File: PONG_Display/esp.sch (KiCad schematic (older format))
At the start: 2 parts, among them J7 ESP_Conn, J8 ESP_Prog_Conn

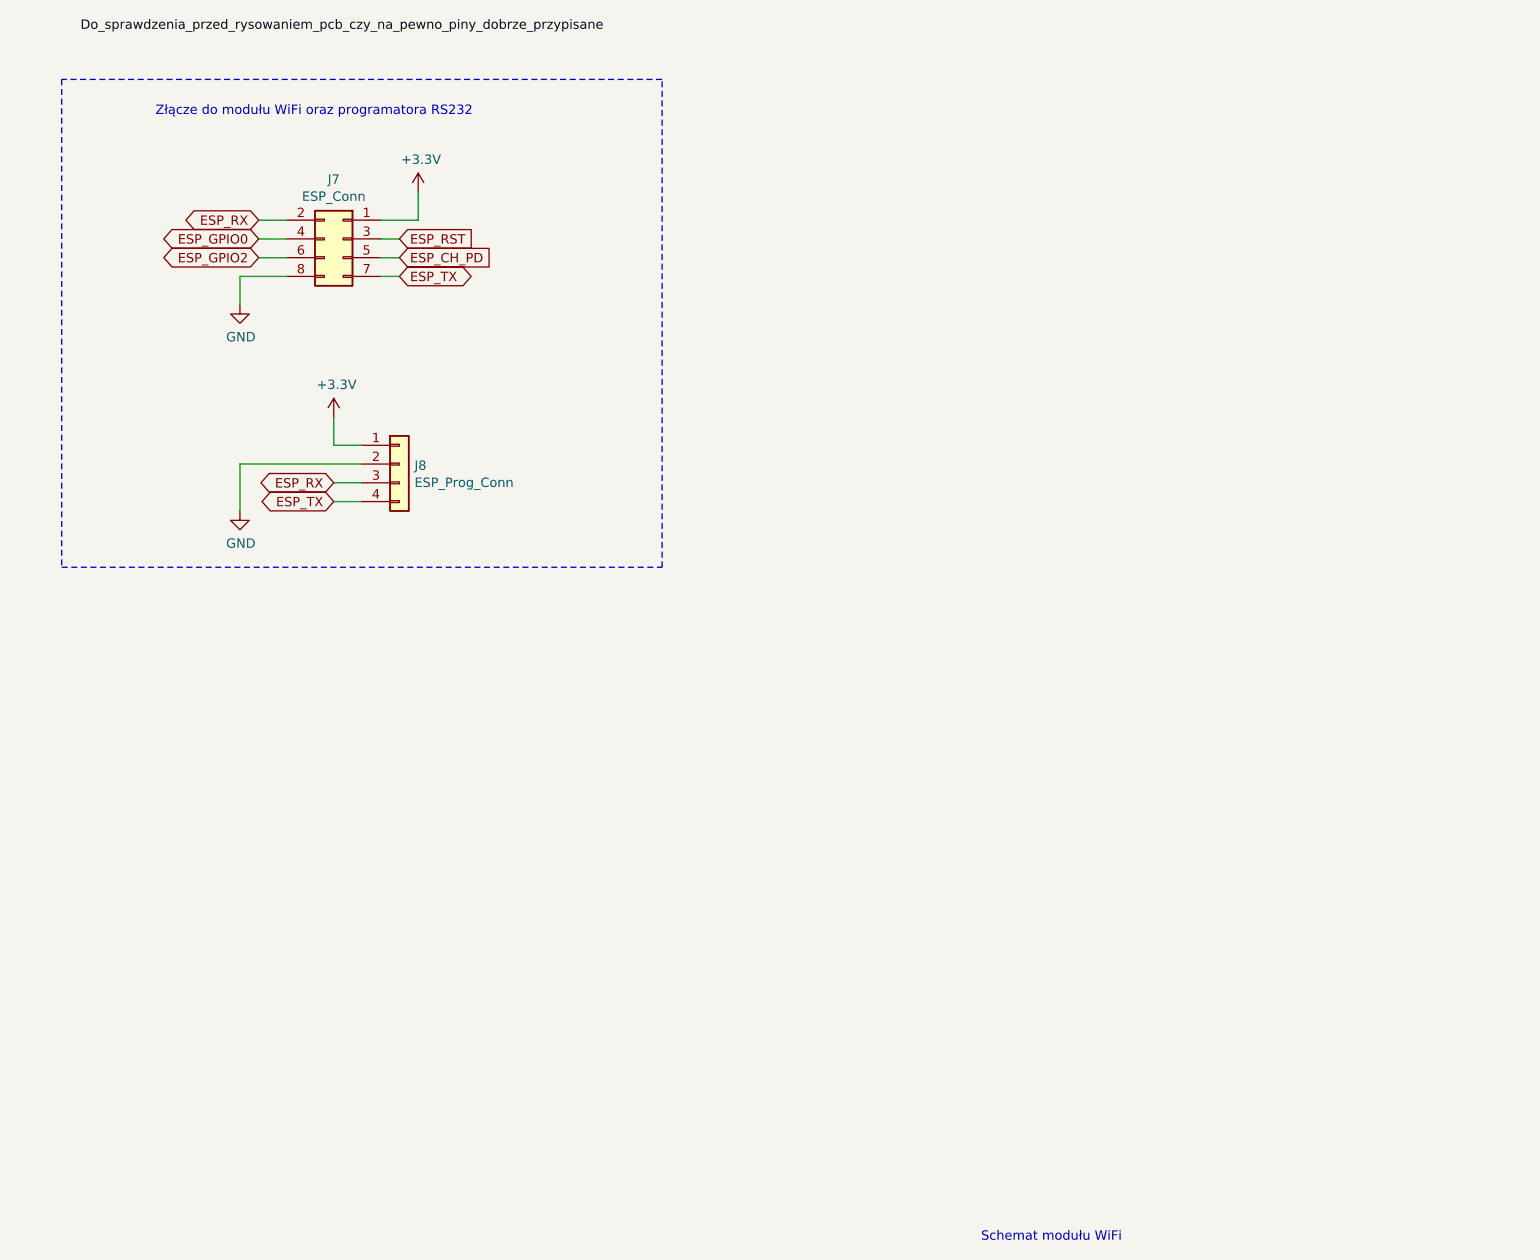
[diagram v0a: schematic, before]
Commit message: Zmiany
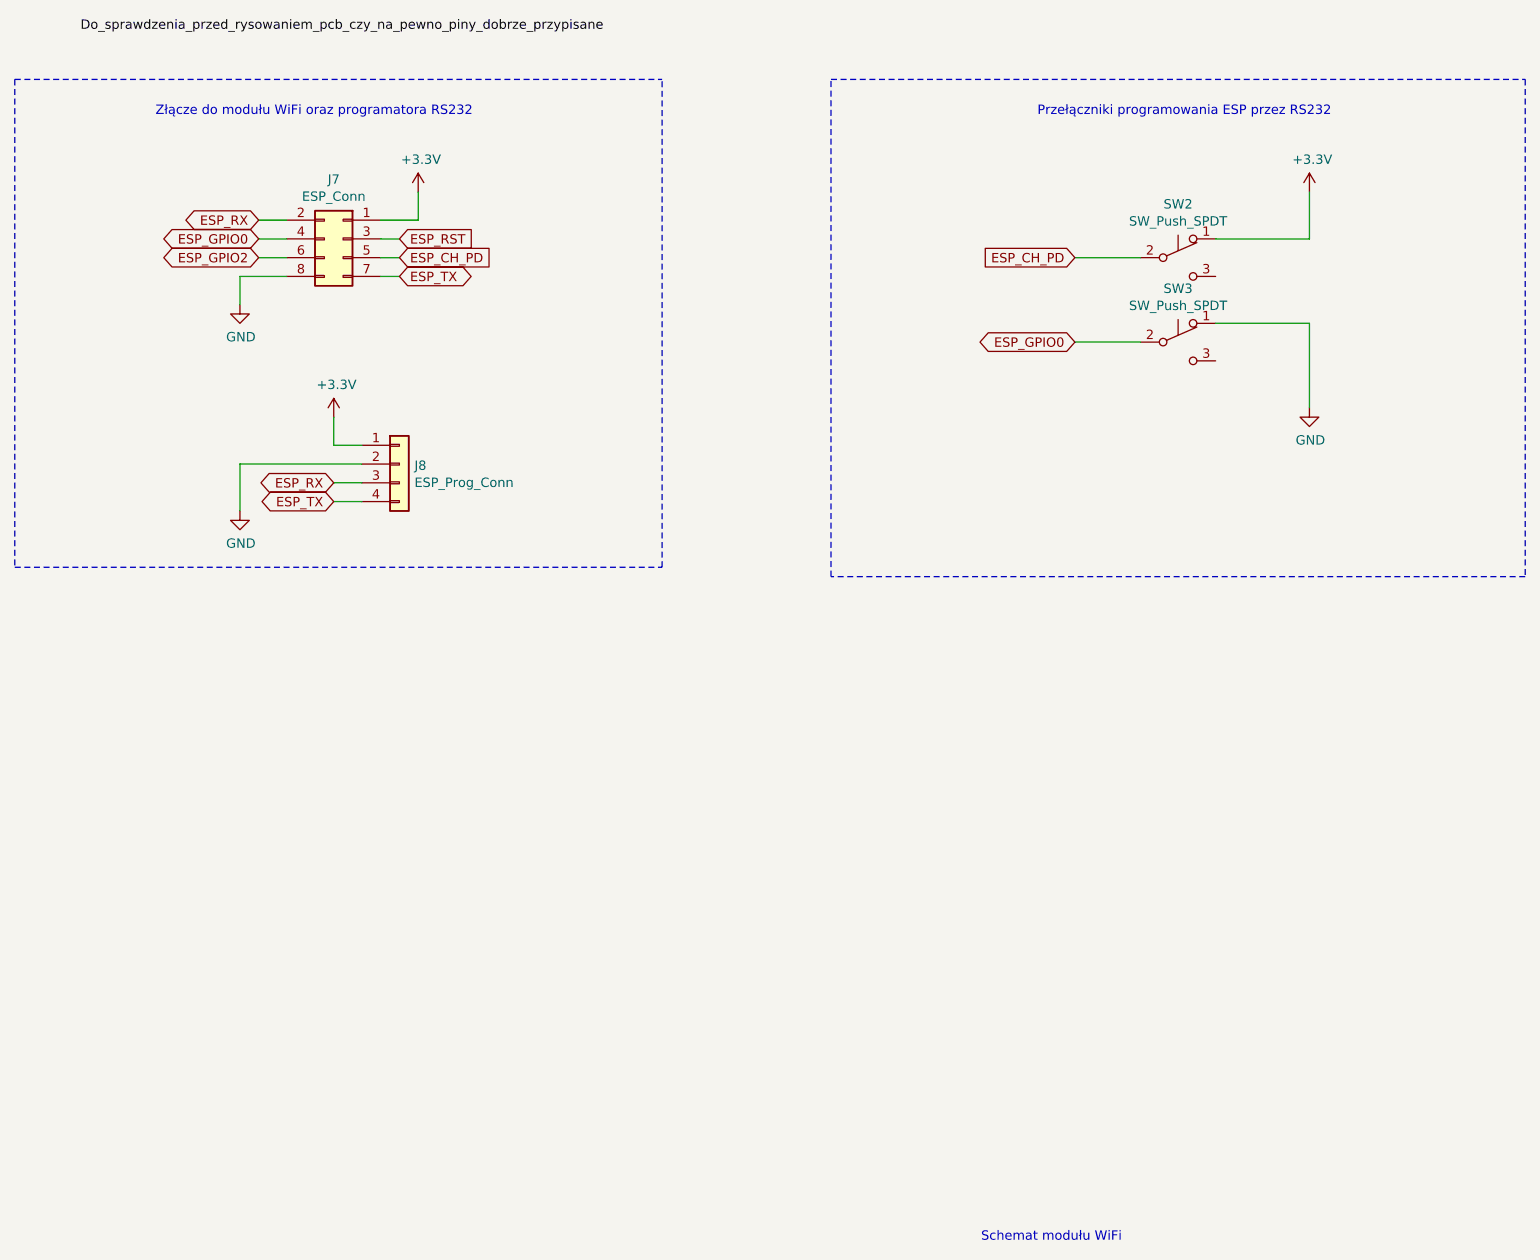
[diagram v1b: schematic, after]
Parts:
- added SW2, SW3: SW_Push_SPDT, LIB_PONG_Display:SPDT_switch, symbol Switch:SW_Push_SPDT
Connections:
- net +3V3: now also SW2.1 (A)
- net ESP_CH_PD: now also SW2.2 (B)
- net ESP_GPIO0: now also SW3.2 (B)
- net GND: now also SW3.1 (A)
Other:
- note added: "Przełączniki programowania ESP przez RS232"
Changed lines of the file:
@@
 	3850 3350 4500 3350
-Wire Notes Line
-	2900 3900 6100 3900
 Wire Notes Line
 	6100 3900 6100 1300
 Wire Notes Line
-	6100 1300 2900 1300
-Wire Notes Line
-	2900 1300 2900 3900
+	2650 1300 2650 3900
 Text Notes 3400 1500 0    50   ~ 0
 Złącze do modułu WiFi oraz programatora RS232
 Text Label 3000 1050 0    50   ~ 0
 Do_sprawdzenia_przed_rysowaniem_pcb_czy_na_pewno_piny_dobrze_przypisane
+Wire Notes Line
+	2650 1300 6100 1300
+Wire Notes Line
+	2650 3900 6100 3900
+Wire Notes Line
+	10700 1300 10700 3950
+Wire Notes Line
+	10700 3950 7000 3950
+Wire Notes Line
+	7000 3950 7000 1300
+Wire Notes Line
+	7000 1300 10700 1300
+Text Notes 8100 1500 0    50   ~ 0
+Przełączniki programowania ESP przez RS232
+Text GLabel 8300 2250 0    50   Input ~ 0
+ESP_CH_PD
+Text GLabel 8300 2700 0    50   BiDi ~ 0
+ESP_GPIO0
+$Comp
+L power:+3.3V #PWR01
+U 1 1 5E9D6E89
+P 9550 1900
+F 0 "#PWR01" H 9550 1750 50  0001 C CNN
+F 1 "+3.3V" H 9565 2073 50  0000 C CNN
+F 2 "" H 9550 1900 50  0001 C CNN
+F 3 "" H 9550 1900 50  0001 C CNN
+	1    9550 1900
+	1    0    0    -1
+$EndComp
+$Comp
+L power:GND #PWR02
+U 1 1 5E9D779A
+P 9550 3050
+F 0 "#PWR02" H 9550 2800 50  0001 C CNN
+F 1 "GND" H 9555 2877 50  0000 C CNN
+F 2 "" H 9550 3050 50  0001 C CNN
+F 3 "" H 9550 3050 50  0001 C CNN
+	1    9550 3050
+	1    0    0    -1
+$EndComp
+Wire Wire Line
+	9550 1900 9550 2150
+Wire Wire Line
+	9550 2150 9050 2150
+Wire Wire Line
+	9050 2600 9550 2600
+Wire Wire Line
+	9550 2600 9550 3050
+Wire Wire Line
+	8300 2250 8650 2250
+Wire Wire Line
+	8300 2700 8650 2700
+$Comp
+L Switch:SW_Push_SPDT SW2
+U 1 1 5E9E35EF
+P 8850 2250
+F 0 "SW2" H 8850 2535 50  0000 C CNN
+F 1 "SW_Push_SPDT" H 8850 2444 50  0000 C CNN
+F 2 "LIB_PONG_Display:SPDT_switch" H 8850 2250 50  0001 C CNN
+F 3 "~" H 8850 2250 50  0001 C CNN
+	1    8850 2250
+	1    0    0    -1
+$EndComp
+$Comp
+L Switch:SW_Push_SPDT SW3
+U 1 1 5E9E3E9D
+P 8850 2700
+F 0 "SW3" H 8850 2985 50  0000 C CNN
+F 1 "SW_Push_SPDT" H 8850 2894 50  0000 C CNN
+F 2 "LIB_PONG_Display:SPDT_switch" H 8850 2700 50  0001 C CNN
+F 3 "~" H 8850 2700 50  0001 C CNN
+	1    8850 2700
+	1    0    0    -1
+$EndComp
 $EndSCHEMATC

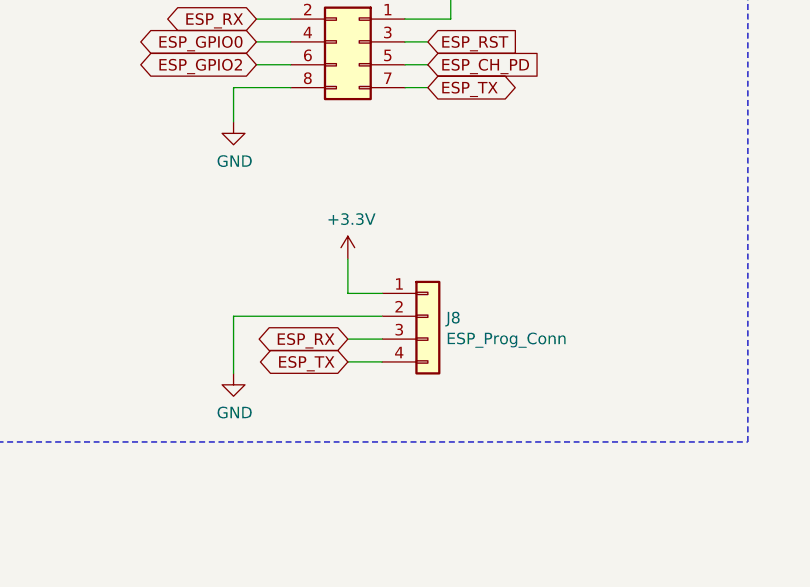
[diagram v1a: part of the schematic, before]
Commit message: Zmiana
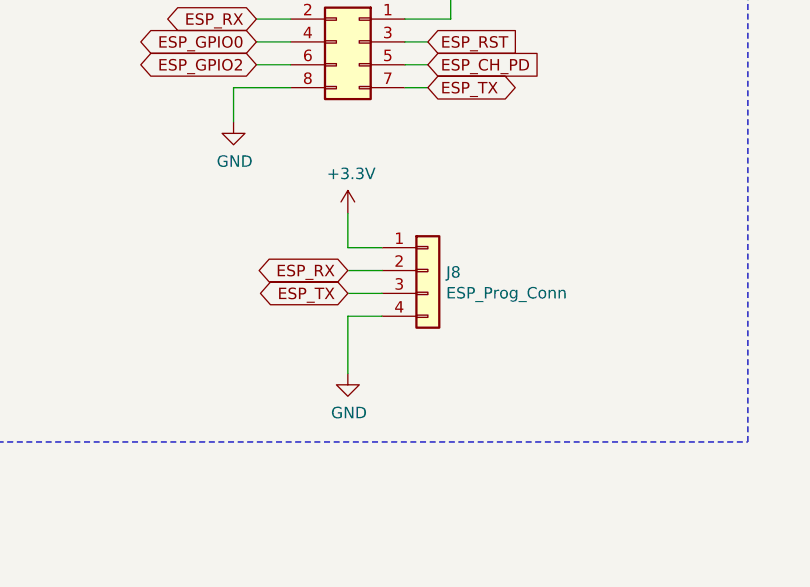
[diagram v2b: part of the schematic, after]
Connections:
- net ESP_RX: now also J8.2 (Pin_2); no longer J8.3 (Pin_3)
- net ESP_TX: now also J8.3 (Pin_3); no longer J8.4 (Pin_4)
- net GND: now also J8.4 (Pin_4); no longer J8.2 (Pin_2)
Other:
- moved on the sheet: J8
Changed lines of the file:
@@
 L Connector_Generic:Conn_01x04 J?
 U 1 1 5E838282
-P 4700 3350
+P 4700 3150
 AR Path="/5E80CCDD/5E838282" Ref="J?"  Part="1"
 AR Path="/5E80B1F8/5E838282" Ref="J8"  Part="1"
-F 0 "J8" H 4780 3342 50  0000 L CNN
-F 1 "ESP_Prog_Conn" H 4780 3251 50  0000 L CNN
-F 2 "Connector_PinHeader_2.54mm:PinHeader_1x04_P2.54mm_Vertical" H 4700 3350 50  0001 C CNN
-F 3 "~" H 4700 3350 50  0001 C CNN
-	1    4700 3350
+F 0 "J8" H 4780 3142 50  0000 L CNN
+F 1 "ESP_Prog_Conn" H 4780 3051 50  0000 L CNN
+F 2 "Connector_PinHeader_2.54mm:PinHeader_1x04_P2.54mm_Vertical" H 4700 3150 50  0001 C CNN
+F 3 "~" H 4700 3150 50  0001 C CNN
+	1    4700 3150
 	1    0    0    -1
 $EndComp
 Wire Wire Line
+	4350 3050 4500 3050
+Wire Wire Line
+	4350 3150 4500 3150
+Wire Wire Line
 	4350 3250 4500 3250
-Wire Wire Line
-	4350 3450 4500 3450
-Wire Wire Line
-	4350 3550 4500 3550
-Text GLabel 4350 3550 0    50   BiDi ~ 0
+Text GLabel 4350 3250 0    50   BiDi ~ 0
 ESP_TX
-Text GLabel 4350 3450 0    50   BiDi ~ 0
+Text GLabel 4350 3150 0    50   BiDi ~ 0
 ESP_RX
 Text Notes 7800 7500 0    50   ~ 0
@@
 L power:+3.3V #PWR0175
 U 1 1 5E859CE6
-P 4350 3100
-F 0 "#PWR0175" H 4350 2950 50  0001 C CNN
-F 1 "+3.3V" H 4365 3273 50  0000 C CNN
-F 2 "" H 4350 3100 50  0001 C CNN
-F 3 "" H 4350 3100 50  0001 C CNN
-	1    4350 3100
+P 4350 2900
+F 0 "#PWR0175" H 4350 2750 50  0001 C CNN
+F 1 "+3.3V" H 4365 3073 50  0000 C CNN
+F 2 "" H 4350 2900 50  0001 C CNN
+F 3 "" H 4350 2900 50  0001 C CNN
+	1    4350 2900
 	1    0    0    -1
 $EndComp
@@
 L power:GND #PWR0176
 U 1 1 5E85A6F5
-P 3850 3600
-F 0 "#PWR0176" H 3850 3350 50  0001 C CNN
-F 1 "GND" H 3855 3427 50  0000 C CNN
-F 2 "" H 3850 3600 50  0001 C CNN
-F 3 "" H 3850 3600 50  0001 C CNN
-	1    3850 3600
+P 4350 3600
+F 0 "#PWR0176" H 4350 3350 50  0001 C CNN
+F 1 "GND" H 4355 3427 50  0000 C CNN
+F 2 "" H 4350 3600 50  0001 C CNN
+F 3 "" H 4350 3600 50  0001 C CNN
+	1    4350 3600
 	1    0    0    -1
 $EndComp
 Wire Wire Line
-	4350 3100 4350 3250
+	4350 2900 4350 3050
 Wire Wire Line
-	3850 3350 3850 3600
+	4350 3350 4350 3600
 Wire Wire Line
-	3850 3350 4500 3350
+	4350 3350 4500 3350
 Wire Notes Line
 	6100 3900 6100 1300

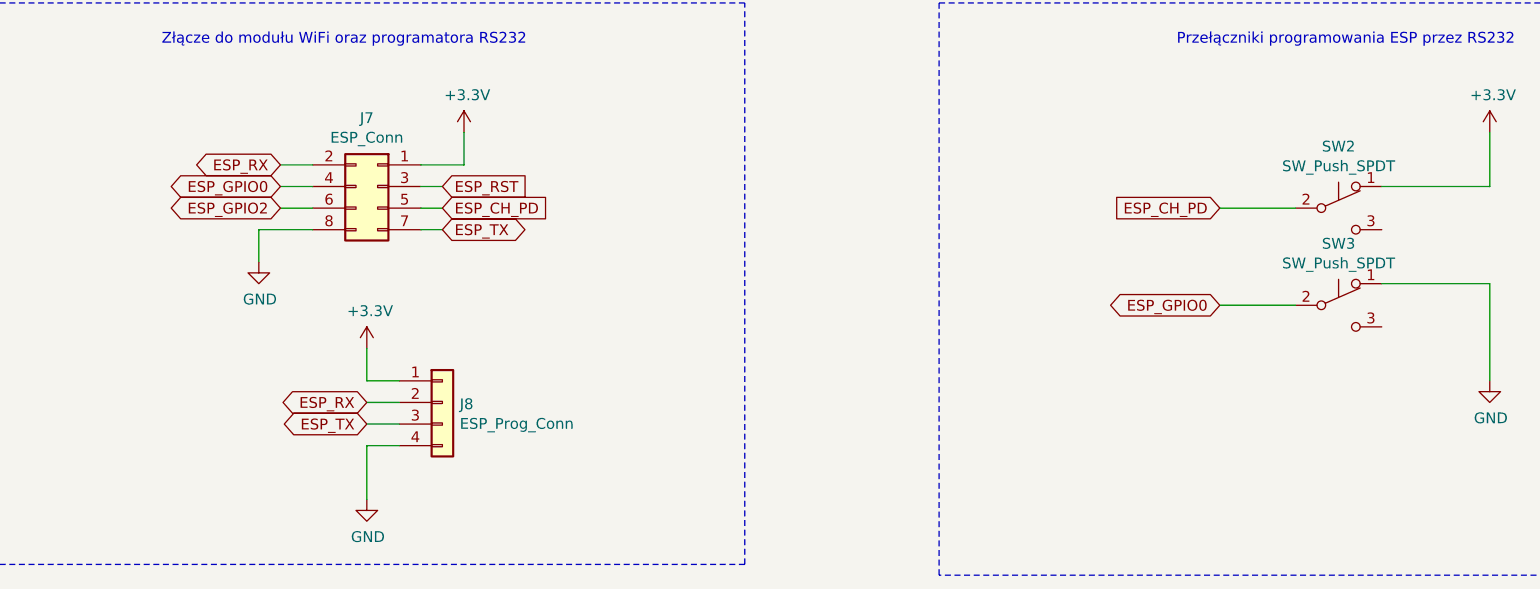
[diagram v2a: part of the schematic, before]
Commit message: Teraz jest sexy
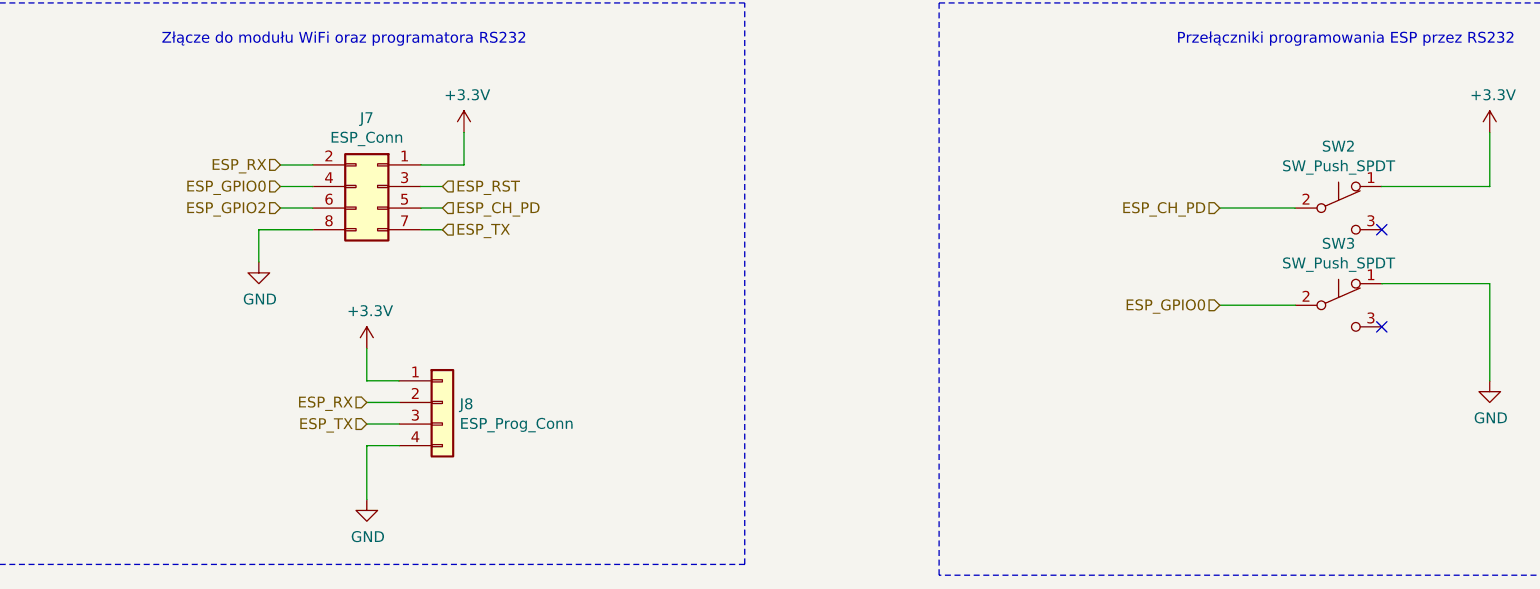
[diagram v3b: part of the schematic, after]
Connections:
- no-connect marks 0 -> 2
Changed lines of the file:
@@
 EESchema Schematic File Version 4
+LIBS:PONG_Display-cache
 EELAYER 30 0
 EELAYER END
@@
 Comment4 ""
 $EndDescr
-Text GLabel 4700 2150 2    50   Input ~ 0
-ESP_RST
-Text GLabel 4700 2250 2    50   Input ~ 0
-ESP_CH_PD
-Text GLabel 4700 2350 2    50   BiDi ~ 0
-ESP_TX
-Text GLabel 3950 2050 0    50   BiDi ~ 0
-ESP_RX
-Text GLabel 3950 2150 0    50   BiDi ~ 0
-ESP_GPIO0
-Text GLabel 3950 2250 0    50   BiDi ~ 0
-ESP_GPIO2
 $Comp
 L Connector_Generic:Conn_02x04_Odd_Even J?
@@
 Wire Wire Line
 	4350 3250 4500 3250
-Text GLabel 4350 3250 0    50   BiDi ~ 0
-ESP_TX
-Text GLabel 4350 3150 0    50   BiDi ~ 0
-ESP_RX
 Text Notes 7800 7500 0    50   ~ 0
 Schemat modułu WiFi
@@
 Text Notes 8100 1500 0    50   ~ 0
 Przełączniki programowania ESP przez RS232
-Text GLabel 8300 2250 0    50   Input ~ 0
-ESP_CH_PD
-Text GLabel 8300 2700 0    50   BiDi ~ 0
-ESP_GPIO0
 $Comp
 L power:+3.3V #PWR01
@@
 	1    0    0    -1
 $EndComp
+Text HLabel 3950 2050 0    50   Input ~ 0
+ESP_RX
+Text HLabel 4700 2350 2    50   Input ~ 0
+ESP_TX
+Text HLabel 4700 2150 2    50   Input ~ 0
+ESP_RST
+Text HLabel 4700 2250 2    50   Input ~ 0
+ESP_CH_PD
+Text HLabel 3950 2150 0    50   Input ~ 0
+ESP_GPIO0
+Text HLabel 3950 2250 0    50   Input ~ 0
+ESP_GPIO2
+Text HLabel 4350 3150 0    50   Input ~ 0
+ESP_RX
+Text HLabel 4350 3250 0    50   Input ~ 0
+ESP_TX
+Text HLabel 8300 2250 0    50   Input ~ 0
+ESP_CH_PD
+Text HLabel 8300 2700 0    50   Input ~ 0
+ESP_GPIO0
+NoConn ~ 9050 2350
+NoConn ~ 9050 2800
 $EndSCHEMATC
